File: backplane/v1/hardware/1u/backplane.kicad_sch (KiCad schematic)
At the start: 14 parts, among them J1 Conn_02x20_Odd_Even, J2 Conn_02x20_Odd_Even, J3 Conn_02x20_Odd_Even, J4 Conn_02x20_Odd_Even

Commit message: finish preliminary 1U design
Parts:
- J1, J2, J3, J4: footprint footprints:SAMTEC_SFM-120-01-L-D-A-TR -> footprints:SFM-120-X1-XXX-D
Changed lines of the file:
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@@
 			)
 		)
-		(property "Footprint" "footprints:SAMTEC_SFM-120-01-L-D-A-TR"
+		(property "Footprint" "footprints:SFM-120-X1-XXX-D"
 			(at 228.6 134.62 0)
 			(hide yes)
@@
 			)
 		)
-		(property "Footprint" "footprints:SAMTEC_SFM-120-01-L-D-A-TR"
+		(property "Footprint" "footprints:SFM-120-X1-XXX-D"
 			(at 68.58 66.04 0)
 			(hide yes)
@@
 			)
 		)
-		(property "Footprint" "footprints:SAMTEC_SFM-120-01-L-D-A-TR"
+		(property "Footprint" "footprints:SFM-120-X1-XXX-D"
 			(at 68.58 134.62 0)
 			(hide yes)
@@
 			)
 		)
-		(property "Footprint" "footprints:SAMTEC_SFM-120-01-L-D-A-TR"
+		(property "Footprint" "footprints:SFM-120-X1-XXX-D"
 			(at 229.87 66.04 0)
 			(hide yes)

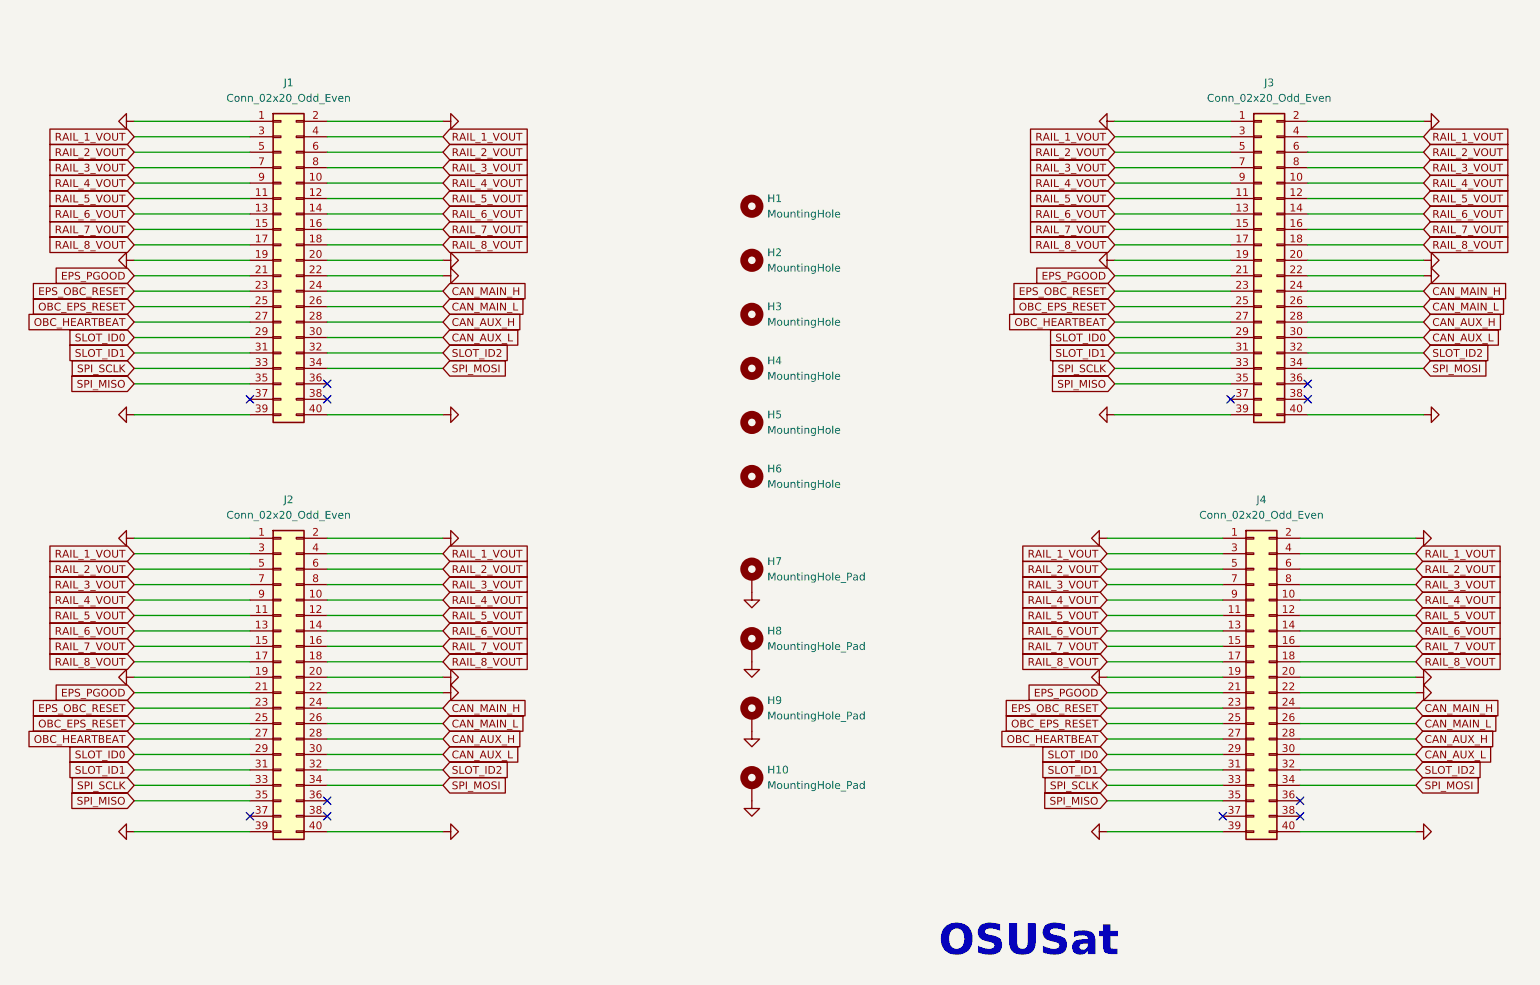
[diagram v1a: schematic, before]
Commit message: revisions from design review
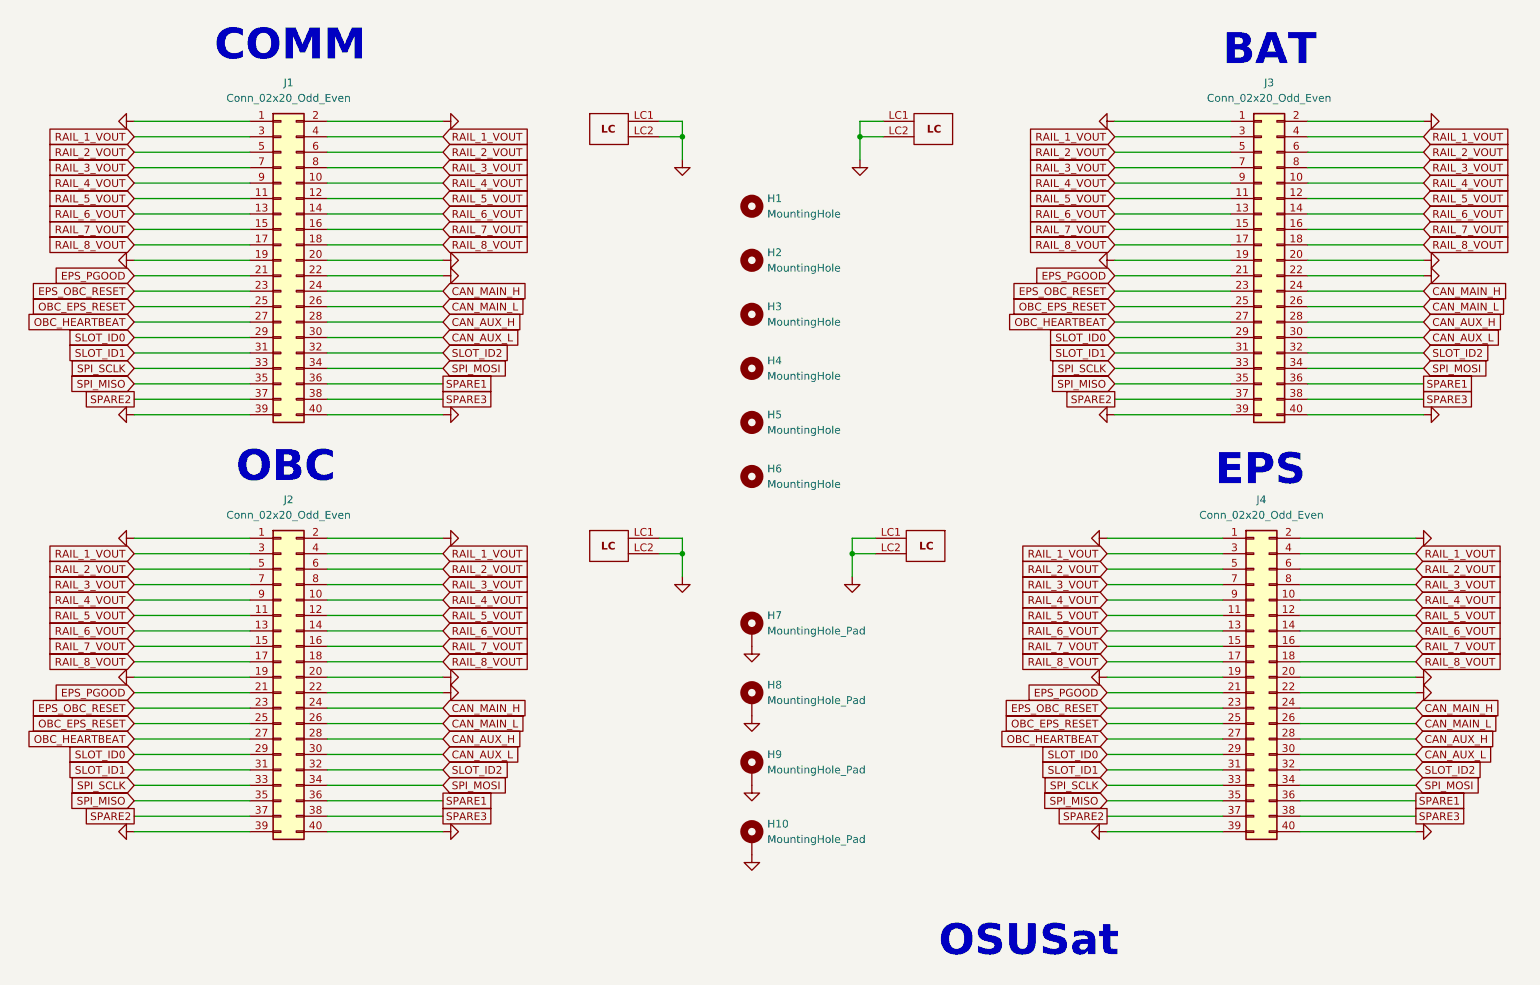
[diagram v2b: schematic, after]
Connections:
- net GND: now also J1.LC1, J1.LC2, J2.LC1, J2.LC2, J3.LC1, J3.LC2, J4.LC1, J4.LC2
- net SPARE1: now reaches J4.36 (Pin_36)
- net SPARE1: now also J1.36 (Pin_36), J2.36 (Pin_36), J3.36 (Pin_36)
- net SPARE2: now reaches J4.37 (Pin_37)
- net SPARE2: now also J1.37 (Pin_37), J2.37 (Pin_37), J3.37 (Pin_37)
- net SPARE3: now reaches J4.38 (Pin_38)
- net SPARE3: now also J1.38 (Pin_38), J2.38 (Pin_38), J3.38 (Pin_38)
- no-connect marks 12 -> 0
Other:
- note added: "BAT"
- note added: "COMM"
- note added: "EPS"
- note added: "OBC"
- moved on the sheet: H10, H7, H8, H9
